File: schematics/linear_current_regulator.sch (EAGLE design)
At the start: 3 parts, among them IC1 LM2931_FIXED

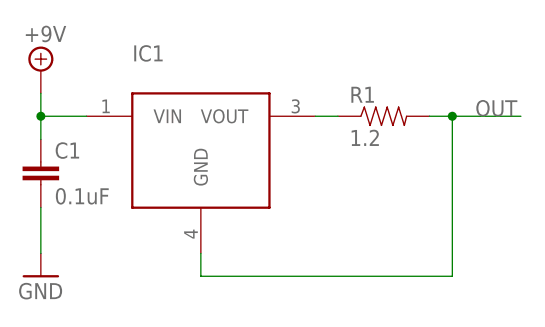
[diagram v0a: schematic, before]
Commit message: Numerous errata
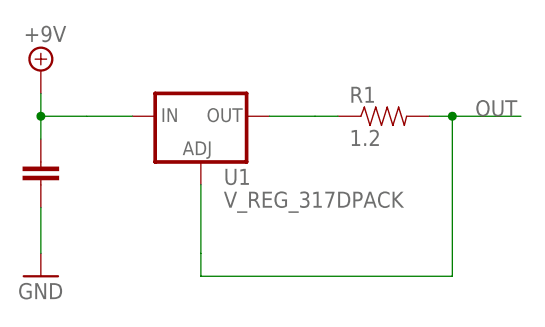
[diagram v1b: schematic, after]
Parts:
- removed IC1: LM2931_FIXED, SparkFun-PowerIC:LM2931_FIXED
- added U1: V_REG_317DPACK, SparkFun-PowerIC:V_REG_317DPACK
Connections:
- net +9V: now also U1.IN; no longer IC1.VIN
- net N$1: now also U1.OUT; no longer IC1.VOUT
- net OUT: now also U1.ADJ; no longer IC1.GND
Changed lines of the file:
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@@
 </classes>
 <parts>
-<part name="IC1" library="SparkFun-PowerIC" deviceset="LM2931_FIXED" device="" value=""/>
 <part name="SUPPLY1" library="supply2" deviceset="+9V" device=""/>
 <part name="C1" library="SparkFun-Passives" deviceset="CAP" device="0402-CAP" value="0.1uF"/>
 <part name="R1" library="SparkFun-Passives" deviceset="RESISTOR" device="0402-RES" value="1.2"/>
 <part name="GND1" library="supply1" deviceset="GND" device=""/>
+<part name="U1" library="SparkFun-PowerIC" deviceset="V_REG_317" device="DPACK"/>
 </parts>
 <sheets>
@@
 </plain>
 <instances>
-<instance part="IC1" gate="G$1" x="53.34" y="40.64"/>
 <instance part="SUPPLY1" gate="G$1" x="35.56" y="48.26"/>
-<instance part="C1" gate="G$1" x="35.56" y="35.56"/>
+<instance part="C1" gate="G$1" x="35.56" y="35.56" smashed="yes"/>
 <instance part="R1" gate="G$1" x="73.66" y="43.18"/>
 <instance part="GND1" gate="1" x="35.56" y="25.4"/>
+<instance part="U1" gate="G$1" x="53.34" y="43.18"/>
 </instances>
 <busses>
@@
 <net name="N$1" class="0">
 <segment>
-<pinref part="IC1" gate="G$1" pin="VOUT"/>
 <pinref part="R1" gate="G$1" pin="1"/>
 <wire x1="66.04" y1="43.18" x2="68.58" y2="43.18" width="0.1524" layer="91"/>
+<pinref part="U1" gate="G$1" pin="OUT"/>
+<wire x1="60.96" y1="43.18" x2="66.04" y2="43.18" width="0.1524" layer="91"/>
 </segment>
 </net>
@@
 <wire x1="81.28" y1="43.18" x2="81.28" y2="25.4" width="0.1524" layer="91"/>
 <junction x="81.28" y="43.18"/>
-<pinref part="IC1" gate="G$1" pin="GND"/>
 <wire x1="81.28" y1="25.4" x2="53.34" y2="25.4" width="0.1524" layer="91"/>
 <wire x1="53.34" y1="25.4" x2="53.34" y2="27.94" width="0.1524" layer="91"/>
 <label x="83.82" y="43.18" size="1.778" layer="95"/>
+<pinref part="U1" gate="G$1" pin="ADJ"/>
+<wire x1="53.34" y1="35.56" x2="53.34" y2="27.94" width="0.1524" layer="91"/>
 </segment>
 </net>
 <net name="+9V" class="0">
 <segment>
-<pinref part="IC1" gate="G$1" pin="VIN"/>
 <pinref part="SUPPLY1" gate="G$1" pin="+9V"/>
 <wire x1="40.64" y1="43.18" x2="35.56" y2="43.18" width="0.1524" layer="91"/>
@@
 <wire x1="35.56" y1="43.18" x2="35.56" y2="40.64" width="0.1524" layer="91"/>
 <junction x="35.56" y="43.18"/>
+<pinref part="U1" gate="G$1" pin="IN"/>
+<wire x1="40.64" y1="43.18" x2="45.72" y2="43.18" width="0.1524" layer="91"/>
 </segment>
 </net>
